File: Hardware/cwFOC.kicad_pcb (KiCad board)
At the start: 2 copper layers, 46 x 46 mm, 59 parts, among them J1 Motor, J2 Conn_01x06_MountingPin, J3 KF2EDGV, U1 MP6540, U2 AS5600, U3 HT7533, U5 MAX3485, U6 CW32F030K8

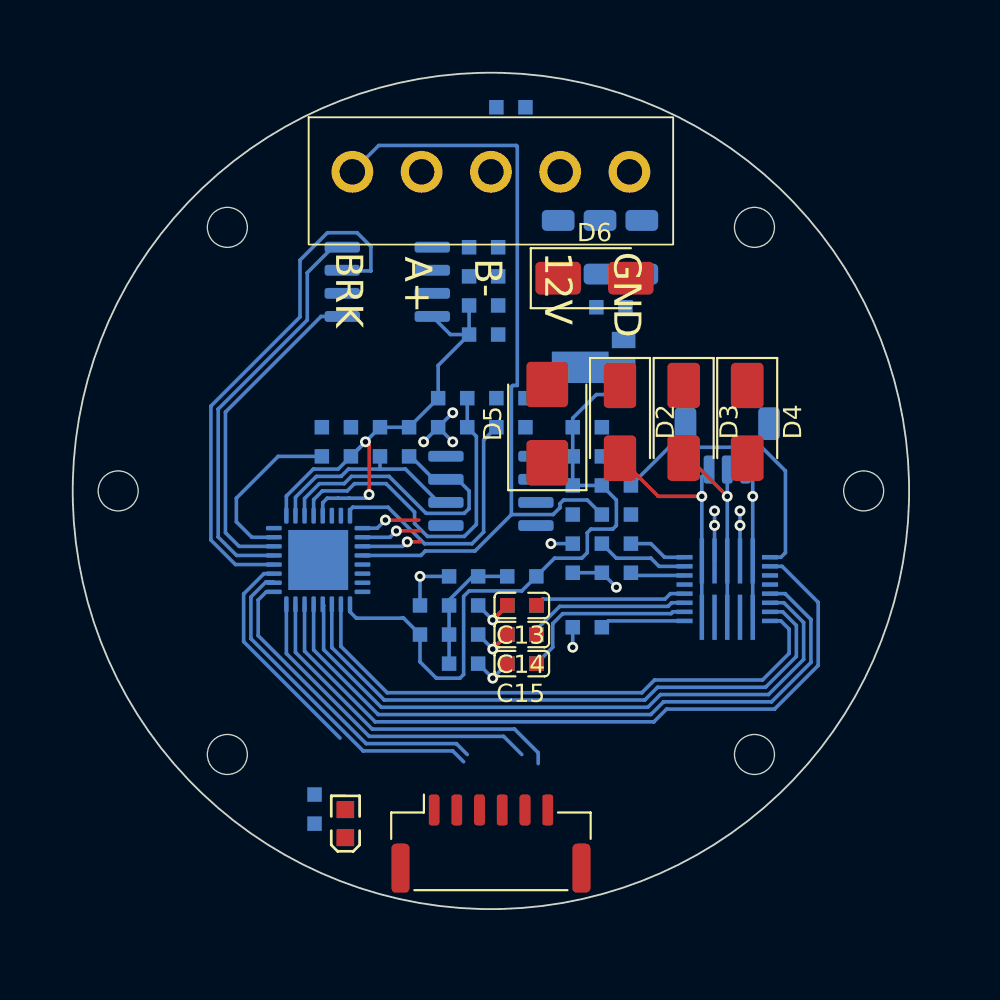
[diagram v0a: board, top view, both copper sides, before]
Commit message: 完成第二版硬件
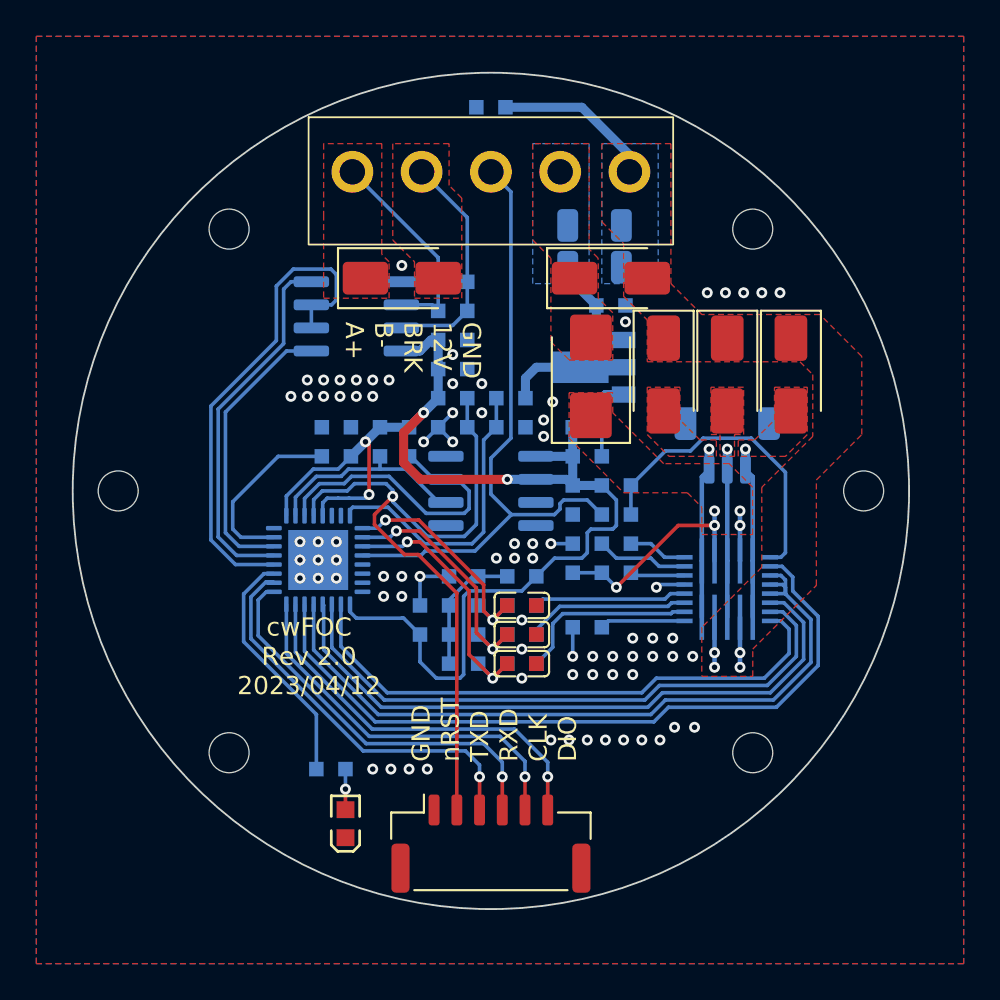
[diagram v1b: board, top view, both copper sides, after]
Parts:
- removed C9: 10uF, Capacitor_SMD:C_1206_3216Metric
- added D7: SMAJ15CA, Diode_SMD:D_SMA, F.Cu at (135.1, 78.3)
- H1, H2, H3, H4, H5, H6: value MountingHole_Pad -> MountingHole; moved to F.Cu
- R3, R4: value 4.7K -> 2.2K
- moved H5 40.9 mm to (125.6, 104.4), turned to 0 degrees
- moved H2 40.9 mm to (154.4, 75.6), turned to 0 degrees
- moved H3 15.7 mm to (160.5, 90.0), turned to 0 degrees
- moved H6 15.7 mm to (119.5, 90.0), turned to 0 degrees
- moved H1 15.6 mm to (125.6, 75.6), turned to 0 degrees
- moved H4 15.6 mm to (154.4, 104.4), turned to 0 degrees
- moved D2 3.54 mm to (149.5, 83.6)
- moved D3 3.54 mm to (153.0, 83.6)
- moved D4 3.54 mm to (156.5, 83.6)
- moved D5 3.54 mm to (145.5, 83.7)
- moved R11 2.55 mm to (138.7, 80.9)
- moved R14 2.55 mm to (137.1, 80.9)
- moved U5 2.55 mm to (132.6, 80.4)
- moved R12 2.55 mm to (137.9, 78.5)
- moved C12 2.55 mm to (137.9, 83.3)
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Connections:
- J2 pad 1: /MCU/SWDIO -> GND
- J2 pad 2: /MCU/SWCLK -> /MCU/nRST
- J2 pad 3: /MCU/RXD -> /MCU/TXD
- J2 pad 4: /MCU/TXD -> /MCU/RXD
- J2 pad 5: /MCU/nRST -> /MCU/SWCLK
- J2 pad 6: GND -> /MCU/SWDIO
- J3 pad 1: BRK -> /RS485/A+
- J3 pad 2: /RS485/A+ -> /RS485/B-
- J3 pad 3: /RS485/B- -> BRK
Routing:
- net /MCU/nRST: track 19.2 -> 39.2 mm, vias 0 -> 1
- net GNDPWR: track 0.00 -> 14.3 mm, vias 0 -> 4
- net VBUS: track 0.00 -> 14.2 mm
- net /RS485/B-: track 0.00 -> 12.7 mm
- net /RS485/A+: track 0.00 -> 11.8 mm
- net /Driver/SOA: track 5.53 -> 15.8 mm
- net BRK: track 45.1 -> 35.2 mm
- net +3V3: track 66.9 -> 75.9 mm, vias 2 -> 4
- net /Driver/SOB: track 6.67 -> 14.8 mm
- net /Driver/SOC: track 6.68 -> 13.9 mm
- net VIN: track 8.23 -> 15.0 mm
- net /MCU/RXD: track 17.2 -> 21.9 mm, vias 0 -> 1
- net /Driver/W: track 13.7 -> 9.42 mm
- net GND: track 8.89 -> 12.6 mm, vias 6 -> 80
- net /MCU/TXD: track 18.4 -> 21.8 mm, vias 0 -> 1
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- added copper zone on F.Cu, net /Driver/U
- added copper zone on F.Cu, net /Driver/V
- added copper zone on F.Cu, net /Driver/W
- added copper zone on F.Cu, net /RS485/A+
- added copper zone on F.Cu, net /RS485/B-
- added copper zone on B.Cu, net GND
- added copper zone on F.Cu, net GND
- added copper zone on B.Cu, net GNDPWR
- added copper zone on F.Cu, net GNDPWR
- added copper zone on B.Cu, net VBUS
- added copper zone on F.Cu, net VBUS
- added copper zone on F.Cu, net VIN
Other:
- board text added: "GND 12V BRK B- A+"
- board text added: "GND nRST TXD RXD CLK DIO"
- board text added: "cwFOC Rev 2.0 2023/04/12"
- board text removed: "12V"
- board text removed: "A+"
- board text removed: "B-"
- board text removed: "BRK"
- board text removed: "GND"
